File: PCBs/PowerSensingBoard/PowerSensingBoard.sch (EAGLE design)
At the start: 38 parts, among them IC1 7805DT, U1 ATTINY84-20SSU

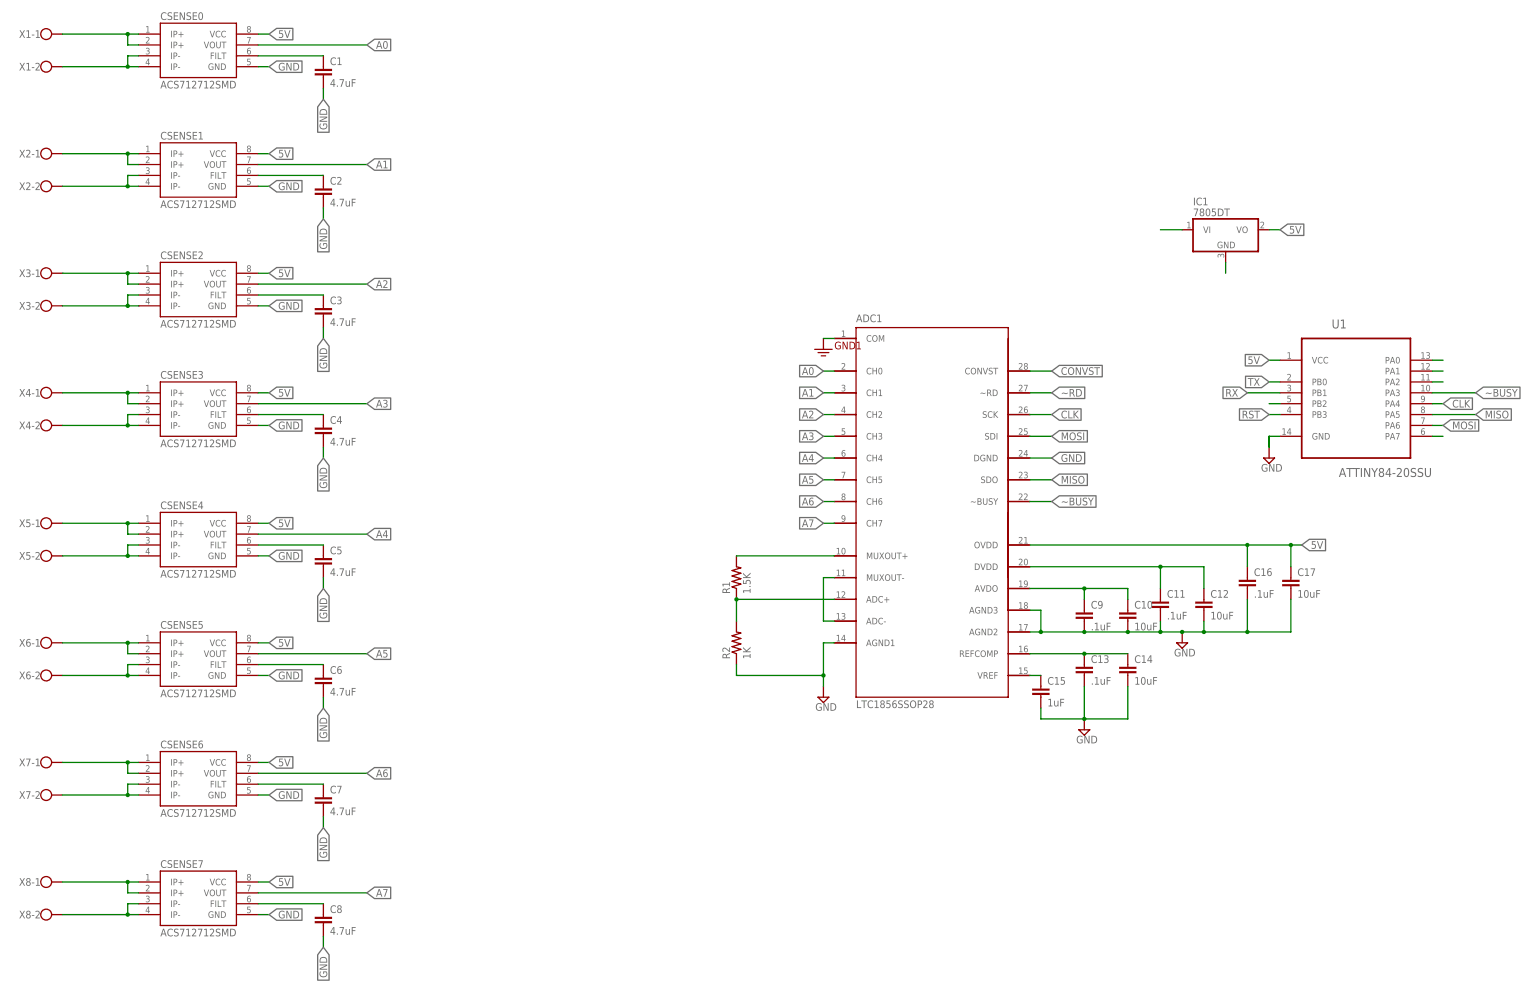
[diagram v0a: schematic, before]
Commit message: Current sensing progress
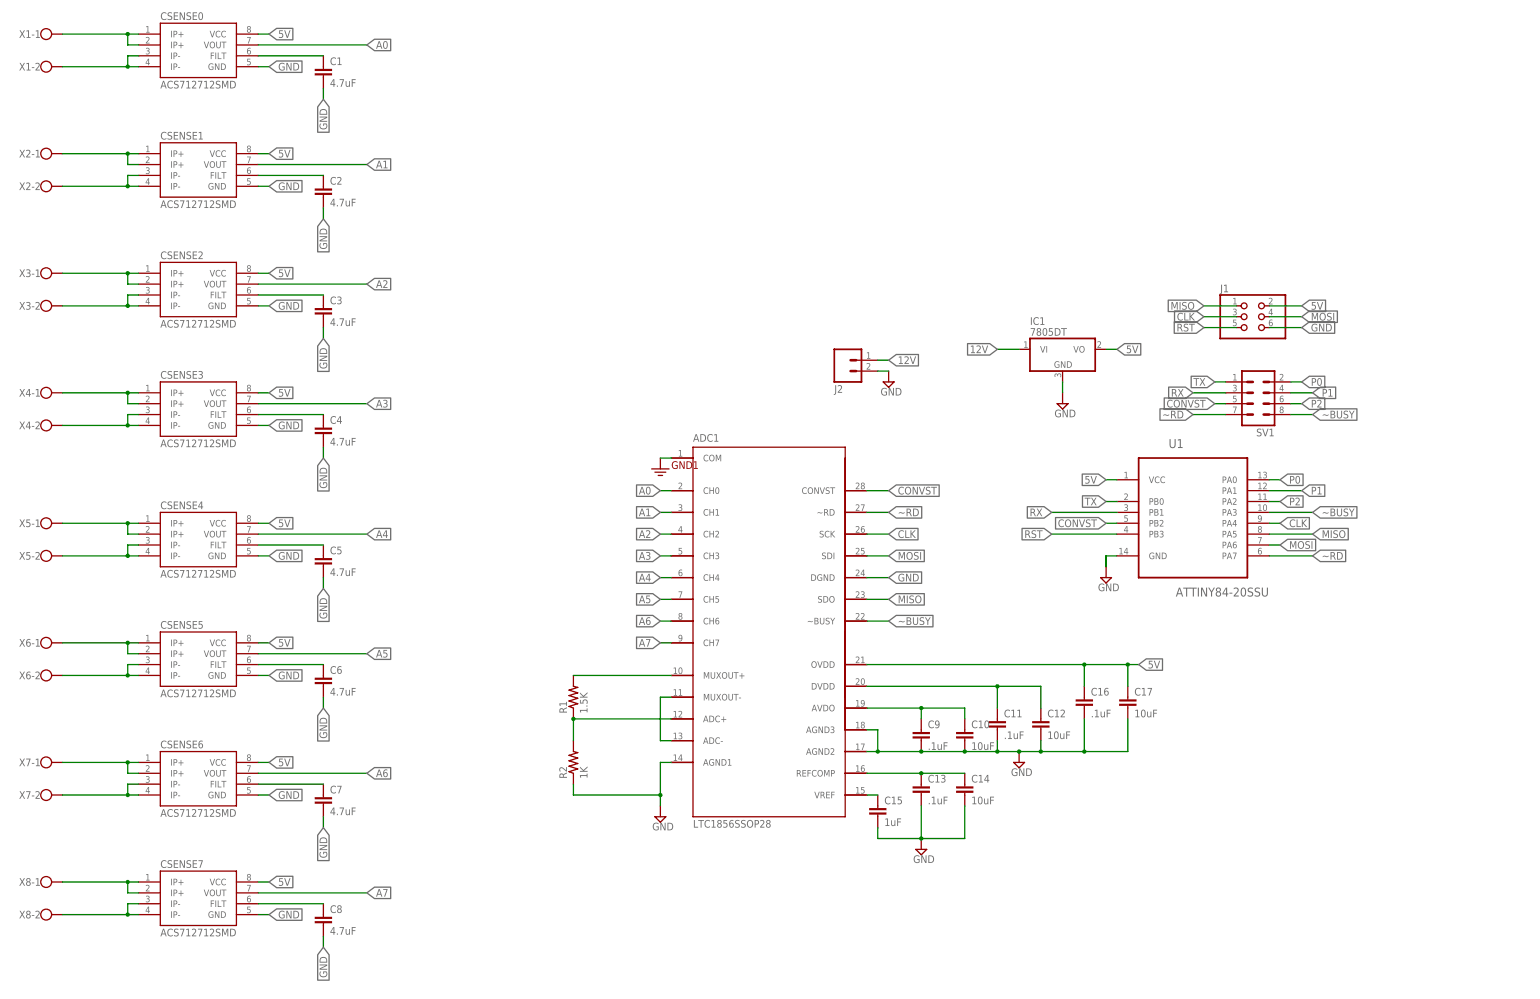
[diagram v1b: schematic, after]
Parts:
- added J1: (no value), SparkFun-Connectors:PINHD-2X3
- added J2: (no value), SparkFun-Connectors:M02PTH
- added SV1: (no value), con-lstb:MA04-2
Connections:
- removed net N$1: U1.PB2
- removed net N$14: U1.PA7
- removed net N$16: IC1.VI
- removed net N$17: IC1.GND
- removed net N$6: U1.PA0
- removed net N$7: U1.PA1
- removed net N$8: U1.PA2
- new net 12V: IC1.VI, J2.1
- new net P0: SV1.2, U1.PA0
- new net P1: SV1.4, U1.PA1
- new net P2: SV1.6, U1.PA2
- net 5V: now also J1.2
- net CLK: now also J1.3
- net CONVST: now also SV1.5, U1.PB2
- net GND: now also IC1.GND, J1.6, J2.2
- net MISO: now also J1.1
- net MOSI: now also J1.4
- net RST: now also J1.5
- net RX: now also SV1.3
- net TX: now also SV1.1
- net ~BUSY: now also SV1.8
- net ~RD: now also SV1.7, U1.PA7
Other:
- moved on the sheet: ADC1, C10, C11, C12, C13, C14, C15, C16, C17, C9, IC1, R1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
